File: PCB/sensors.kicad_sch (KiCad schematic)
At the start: 6 parts, among them J12 R-INMP441, J13 L-INMP441, J15 F_HS-SR04+, J16 B_HS-SR04+, J17 MPU-6050, U12 Module-3

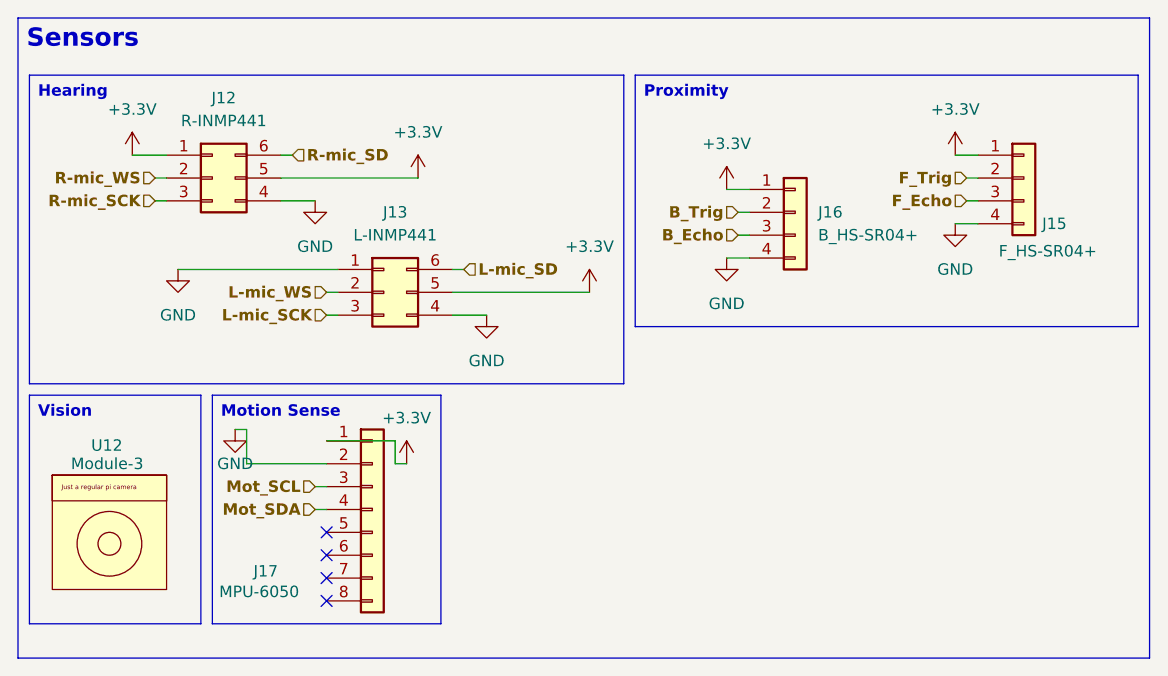
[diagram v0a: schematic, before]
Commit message: [Schem] Finished the whole Schematic (Connected all the pins)
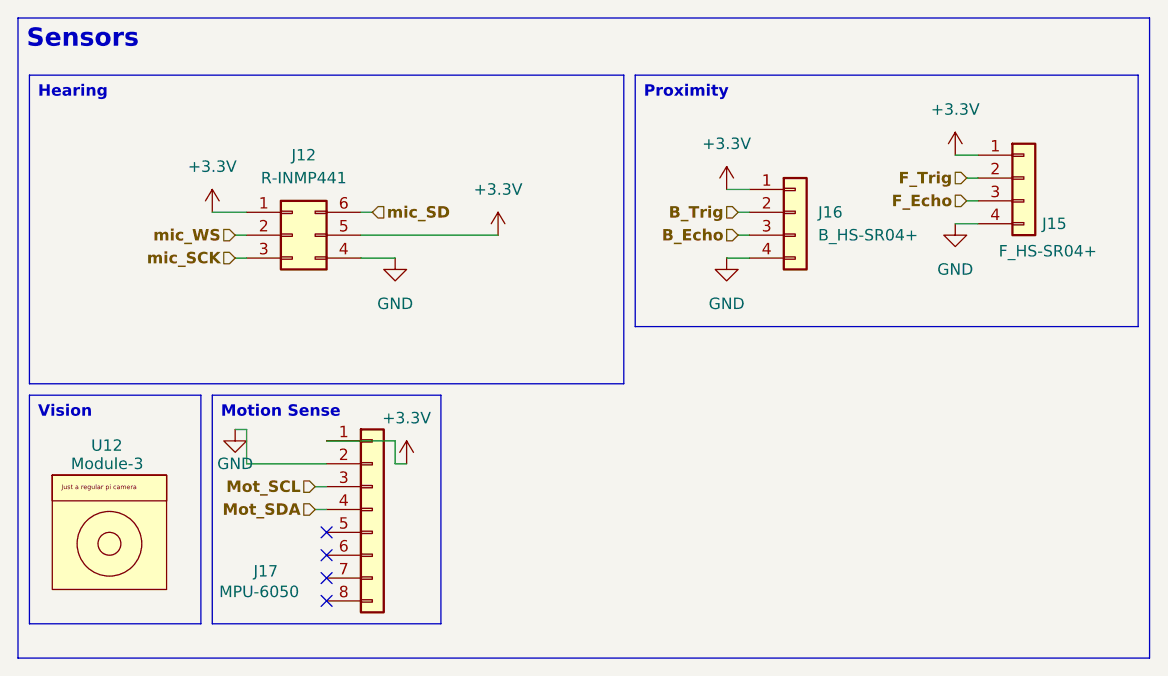
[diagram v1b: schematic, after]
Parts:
- removed J13: L-INMP441, symbol Connector_Generic:Conn_02x03_Counter_Clockwise
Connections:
- net R-mic_SCK renamed mic_SCK
- net R-mic_SD renamed mic_SD
- net R-mic_WS renamed mic_WS
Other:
- moved on the sheet: J12
